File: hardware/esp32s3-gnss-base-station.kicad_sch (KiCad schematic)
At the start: 64 parts, among them CN1 JST 2mm, J1 PWR_BYPASS, J2 OLED, Q1 MMDT3904, SW1 SS-12D10L5, U1 ESP32-S3-WROOM-1-N16R8, U2 ZED-F9P-04B, U3 CP2102-GMR, U4 TP4054, U5 SY8089AAAC, U6 BWMCX-KE

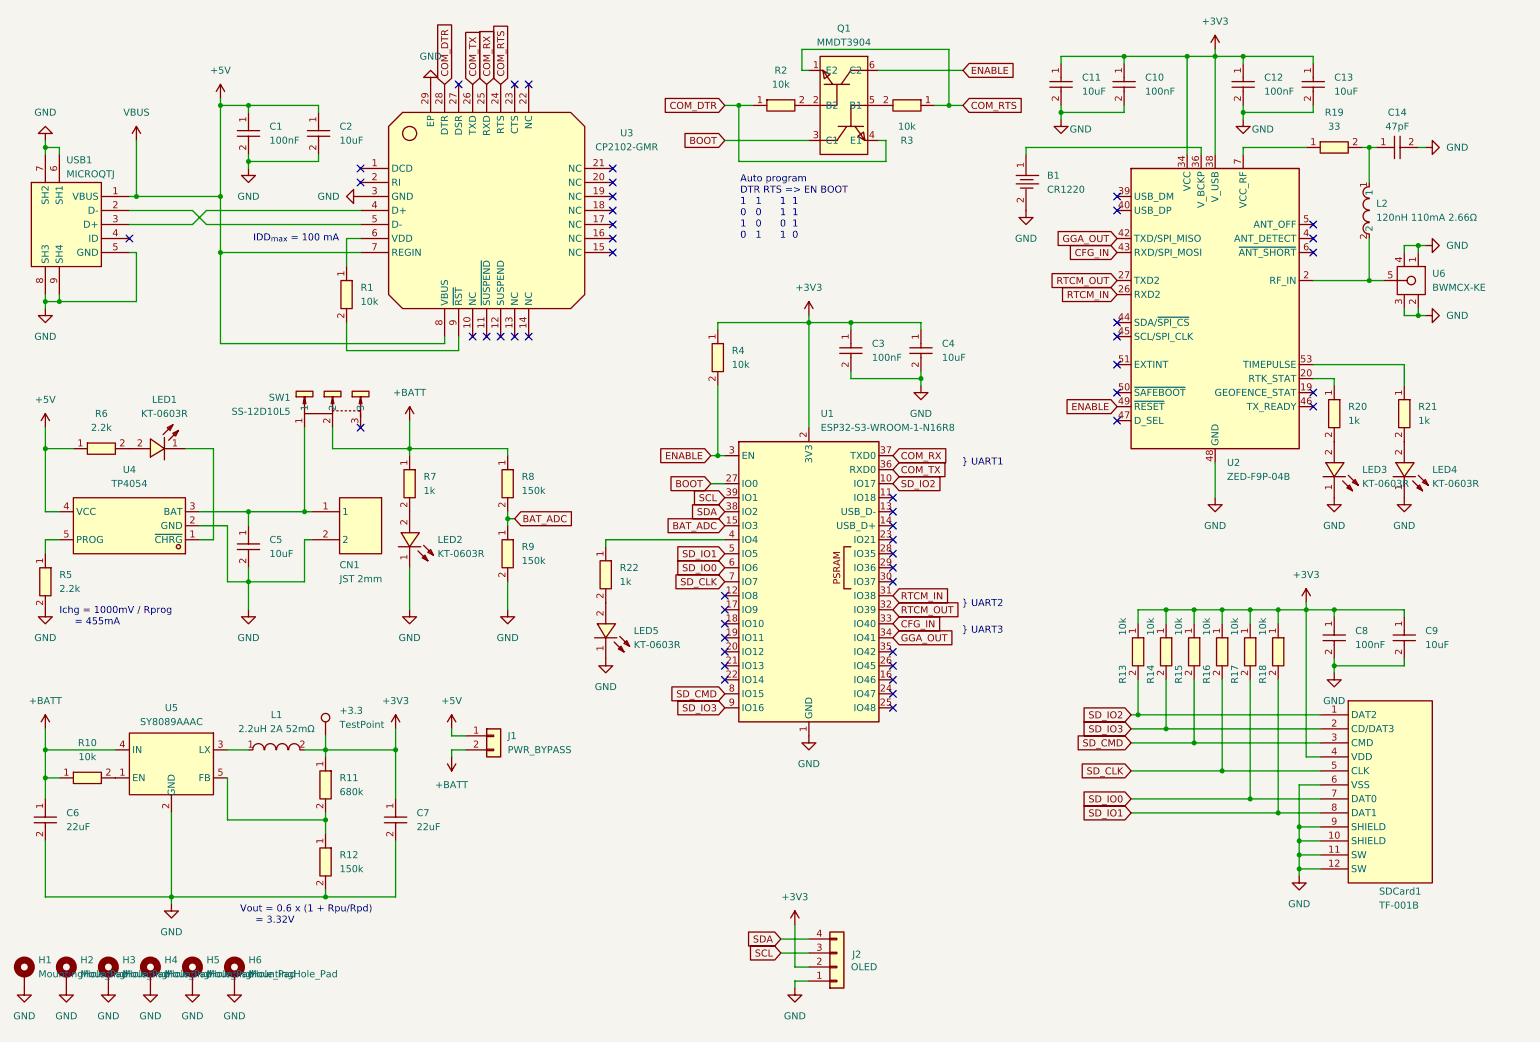
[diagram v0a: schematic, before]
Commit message: Update PCB and export some images
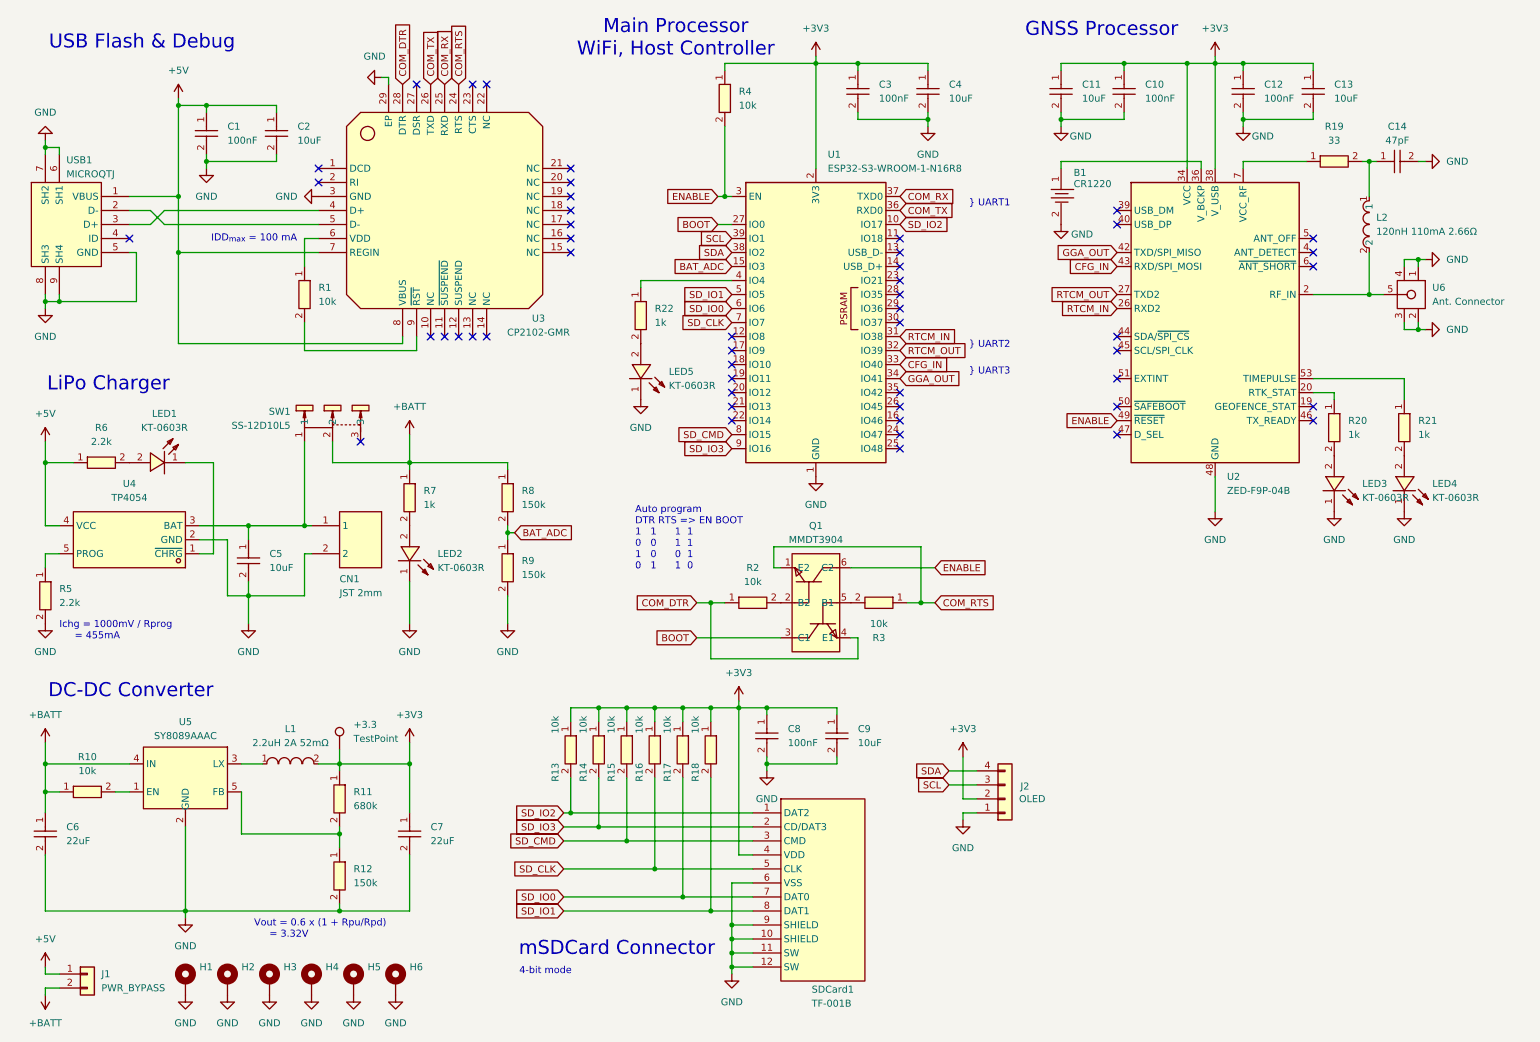
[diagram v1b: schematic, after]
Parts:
- U6: value BWMCX-KE -> Ant. Connector
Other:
- note added: "4-bit mode"
- note added: "DC-DC Converter"
- note added: "GNSS Processor"
- note added: "LiPo Charger"
- note added: "Main Processor WiFi, Host Controller"
- note added: "USB Flash & Debug"
- note added: "mSDCard Connector"
- moved on the sheet: +3.3, B1, C1, C10, C11, C12, C13, C14, C2, C3, C4, C5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
